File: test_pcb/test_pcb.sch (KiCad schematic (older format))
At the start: 91 parts, among them K0 KEYSW, K1 KEYSW, K10 KEYSW, K12 KEYSW, K13 KEYSW, K14 KEYSW, K15 KEYSW, K16 KEYSW, K17 KEYSW, K18 KEYSW, K2 KEYSW, K20 KEYSW, K21 KEYSW, K22 KEYSW, K3 KEYSW, K4 KEYSW, K5 KEYSW, K6 KEYSW, K7 KEYSW, K8 KEYSW, K9 KEYSW, P1 CONN_01X07, P10 CONN_01X01, P11 CONN_01X01, P12 CONN_01X01, P13 CONN_01X01, P14 CONN_01X01, P15 CONN_01X01, P2 CONN_01X07, P3 CONN_01X03, P4 CONN_01X01, P5 CONN_01X01, P6 CONN_01X01, P7 CONN_01X01, P8 CONN_01X01, P9 CONN_01X01, Q0 Si3993CDV, Q1 Si3993CDV, Q2 Si3993CDV, Q3 Si3993CDV, U1 STP16CP05

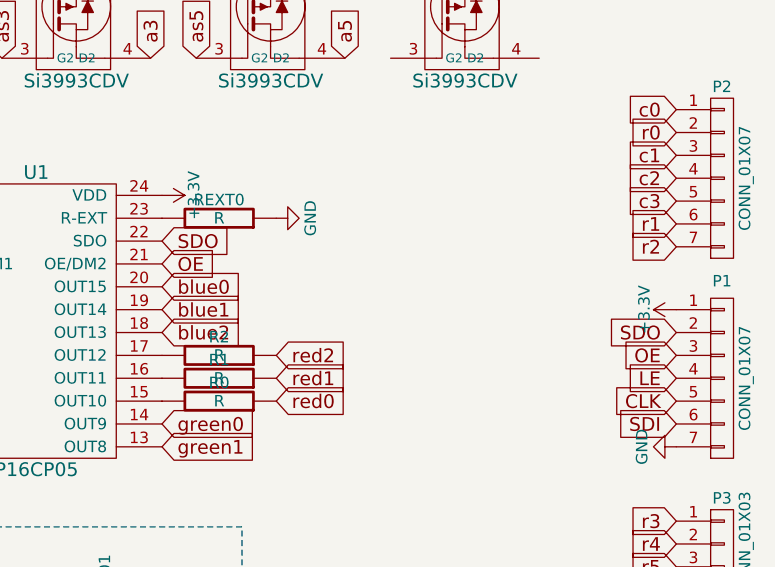
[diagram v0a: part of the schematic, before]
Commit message: test groundplanes
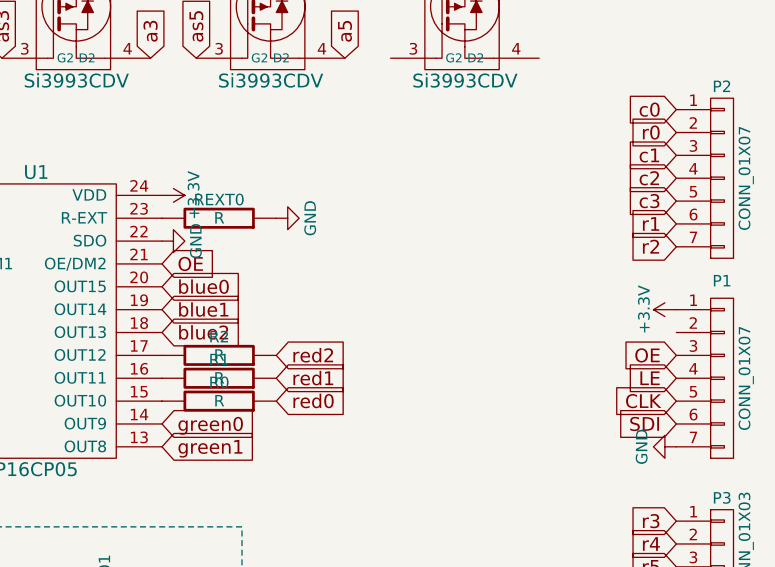
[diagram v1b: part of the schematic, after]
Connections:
- net labels removed: SDO
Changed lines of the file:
@@
 Text GLabel 9850 3600 0    60   Input ~ 0
 LE
-Text GLabel 9850 3400 0    60   Input ~ 0
-SDO
 Text GLabel 9850 3500 0    60   Input ~ 0
 OE
-Text GLabel 7600 3000 2    60   Input ~ 0
-SDO
 Text GLabel 7600 3100 2    60   Input ~ 0
 OE
@@
 	0    1    -1   0
 $EndComp
+$Comp
+L GND #PWR?
+U 1 1 58C10269
+P 7600 3000
+F 0 "#PWR?" H 7600 2750 50  0001 C CNN
+F 1 "GND" H 7600 2850 50  0000 C CNN
+F 2 "" H 7600 3000 50  0000 C CNN
+F 3 "" H 7600 3000 50  0000 C CNN
+	1    7600 3000
+	0    -1   -1   0
+$EndComp
 $EndSCHEMATC
